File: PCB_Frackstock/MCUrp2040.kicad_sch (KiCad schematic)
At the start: 10 parts, among them J2 105450-0101, J3 Conn_01x06_Pin, J4 Conn_01x06_Pin, U1 Pico

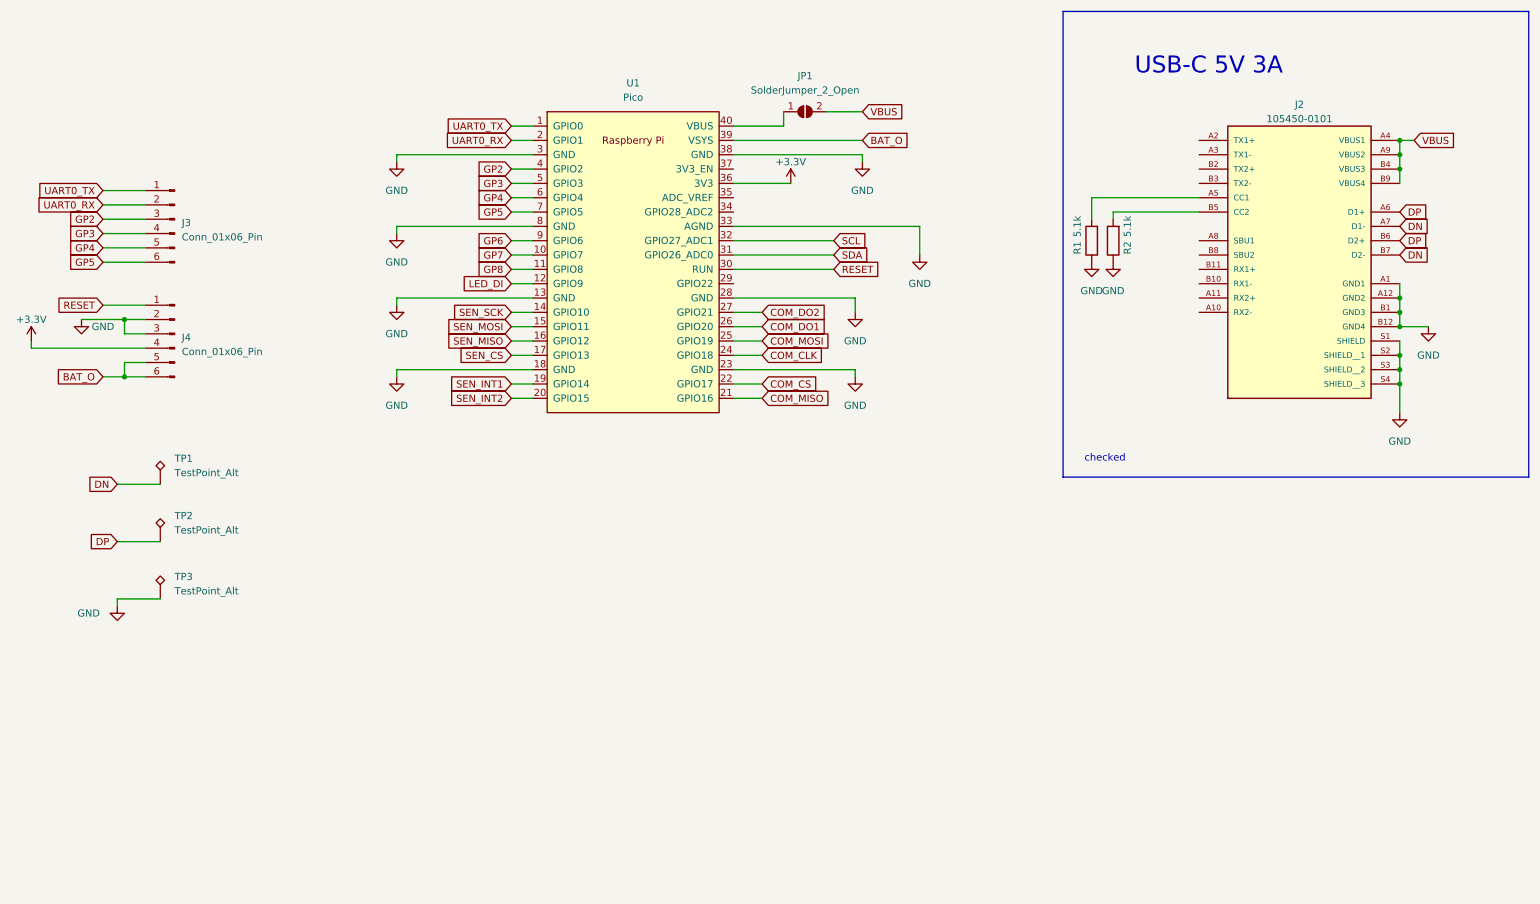
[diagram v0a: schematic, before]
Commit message: Schema-review-1
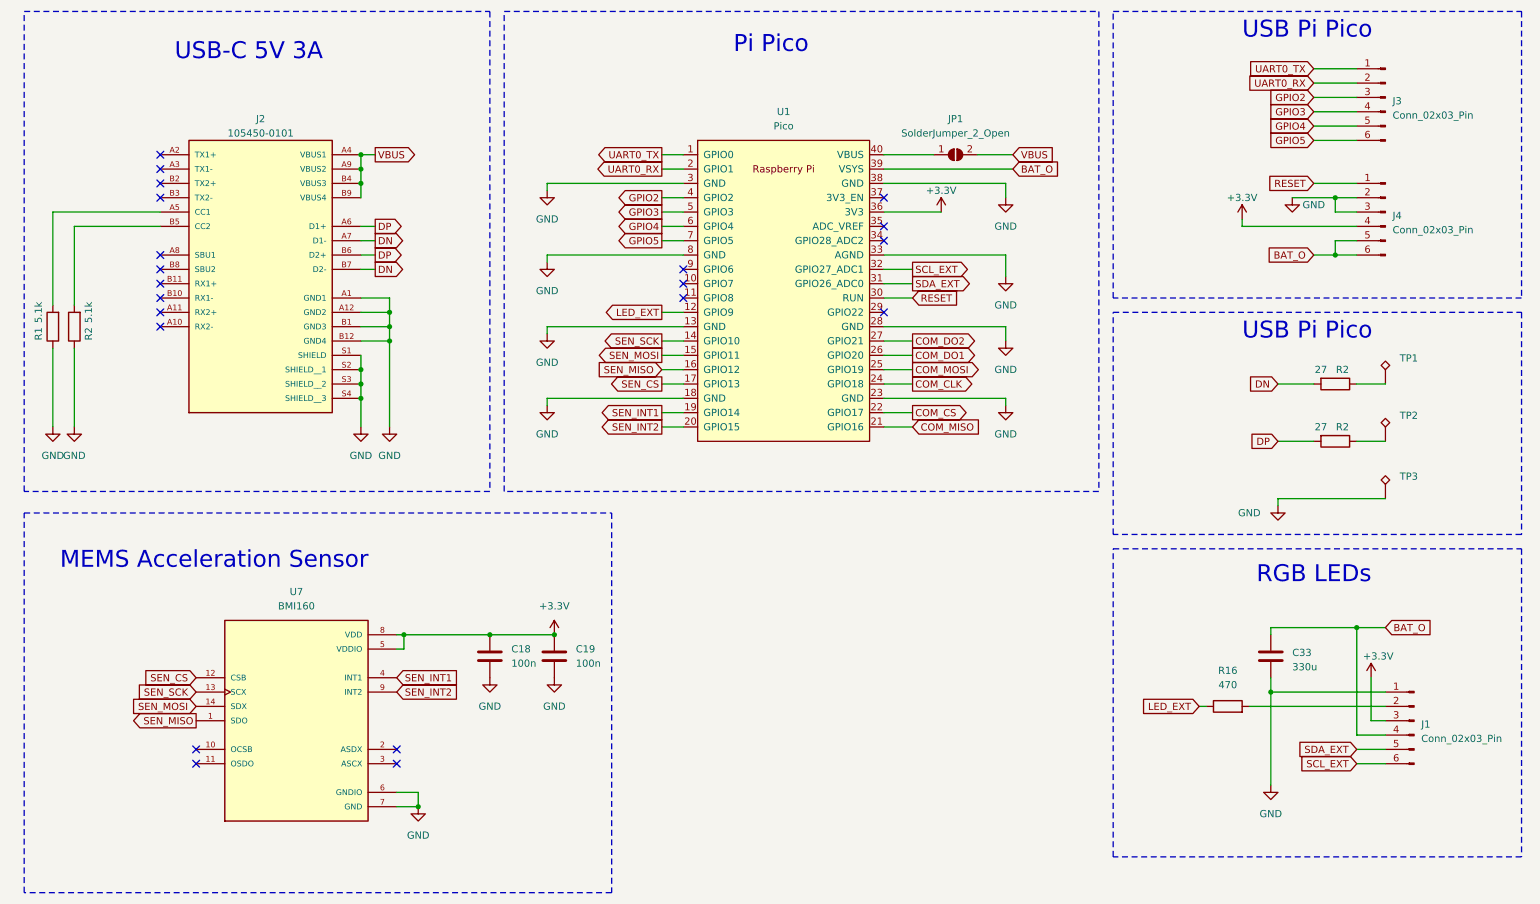
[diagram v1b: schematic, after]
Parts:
- added C18, C19: 100n, Capacitor_SMD:C_0603_1608Metric_Pad1.08x0.95mm_HandSolder, symbol Device:C
- added C33: 330u, Capacitor_SMD:C_0805_2012Metric_Pad1.18x1.45mm_HandSolder, symbol Device:C
- added J1: Conn_02x03_Pin, Frack:PinHeader_2x03_P2.54mm_Vertical_SMD_kleiner, symbol Connector:Conn_01x06_Pin
- added R16: 470, Resistor_SMD:R_0603_1608Metric_Pad0.98x0.95mm_HandSolder, symbol Device:R
- added R2 (x2): 27, Resistor_SMD:R_0603_1608Metric_Pad0.98x0.95mm_HandSolder, symbol Device:R
- added U7: BMI160, Frack:PQFN50P250X300X88-14N, symbol BMI160:BMI160
- J3, J4: value Conn_01x06_Pin -> Conn_02x03_Pin
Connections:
- net +3.3V: now also C18.1, C19.1, J1.3 (Pin_3), U7.5 (VDDIO), U7.8 (VDD)
- net BAT_O: now also C33.2, J1.4 (Pin_4)
- net DN: now also R2.2; no longer TP1.1
- net DP: now also R2.2; no longer TP2.1
- net GND: now also C18.2, C19.2, C33.1, J1.1 (Pin_1), U7.6 (GNDIO), U7.7 (GND)
- net SEN_CS: now also U7.12 (CSB)
- net SEN_INT1: now also U7.4 (INT1)
- net SEN_INT2: now also U7.9 (INT2)
- net SEN_MISO: now also U7.1 (SDO)
- net SEN_MOSI: now also U7.14 (SDX)
- net SEN_SCK: now also U7.13 (SCX)
- net GP2 renamed GPIO2
- net GP3 renamed GPIO3
- net GP4 renamed GPIO4
- net GP5 renamed GPIO5
- net GP6: no longer names the net of U1.9 (GPIO6)
- net GP7: no longer names the net of U1.10 (GPIO7)
- net GP8: no longer names the net of U1.11 (GPIO8)
- net LED_DI renamed LED_EXT
- net LED_EXT: now also R16.1
- net SCL renamed SCL_EXT
- net SCL_EXT: now also J1.6 (Pin_6)
- net SDA renamed SDA_EXT
- net SDA_EXT: now also J1.5 (Pin_5)
- new net: R2.1, TP2.1
- new net: R2.1, TP1.1
- new net: J1.2 (Pin_2), R16.2
- no-connect marks 0 -> 21
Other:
- note added: "MEMS Acceleration Sensor"
- note added: "Pi Pico"
- note added: "RGB LEDs"
- note added: "USB Pi Pico"
- note removed: "checked"
- company: (none) -> Eberkreis
- title: (none) -> Frackstock ET2024
- moved on the sheet: J2, J3, J4, JP1, R1, R2, TP1, TP2, TP3, U1
